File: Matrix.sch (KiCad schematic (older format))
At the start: 210 parts

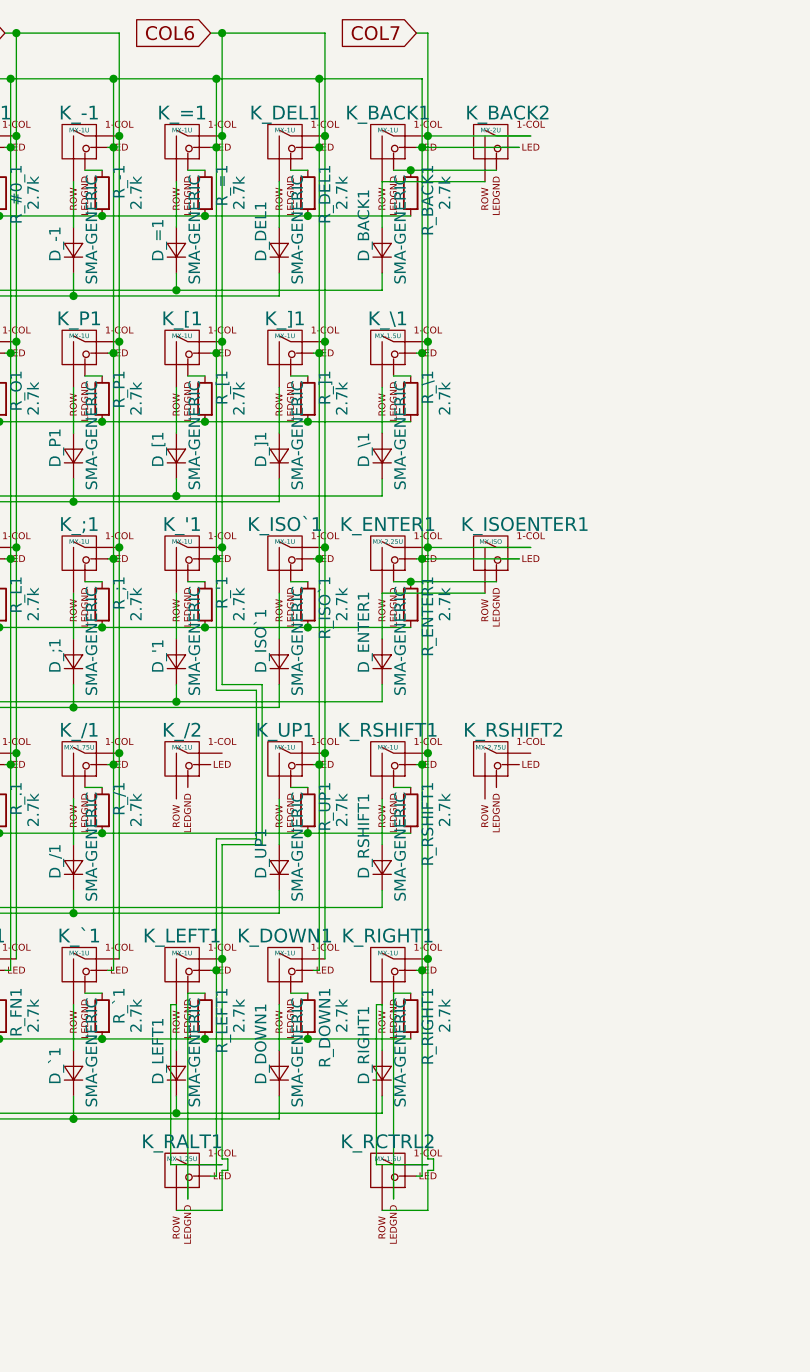
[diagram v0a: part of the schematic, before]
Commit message: Wire more LEDs
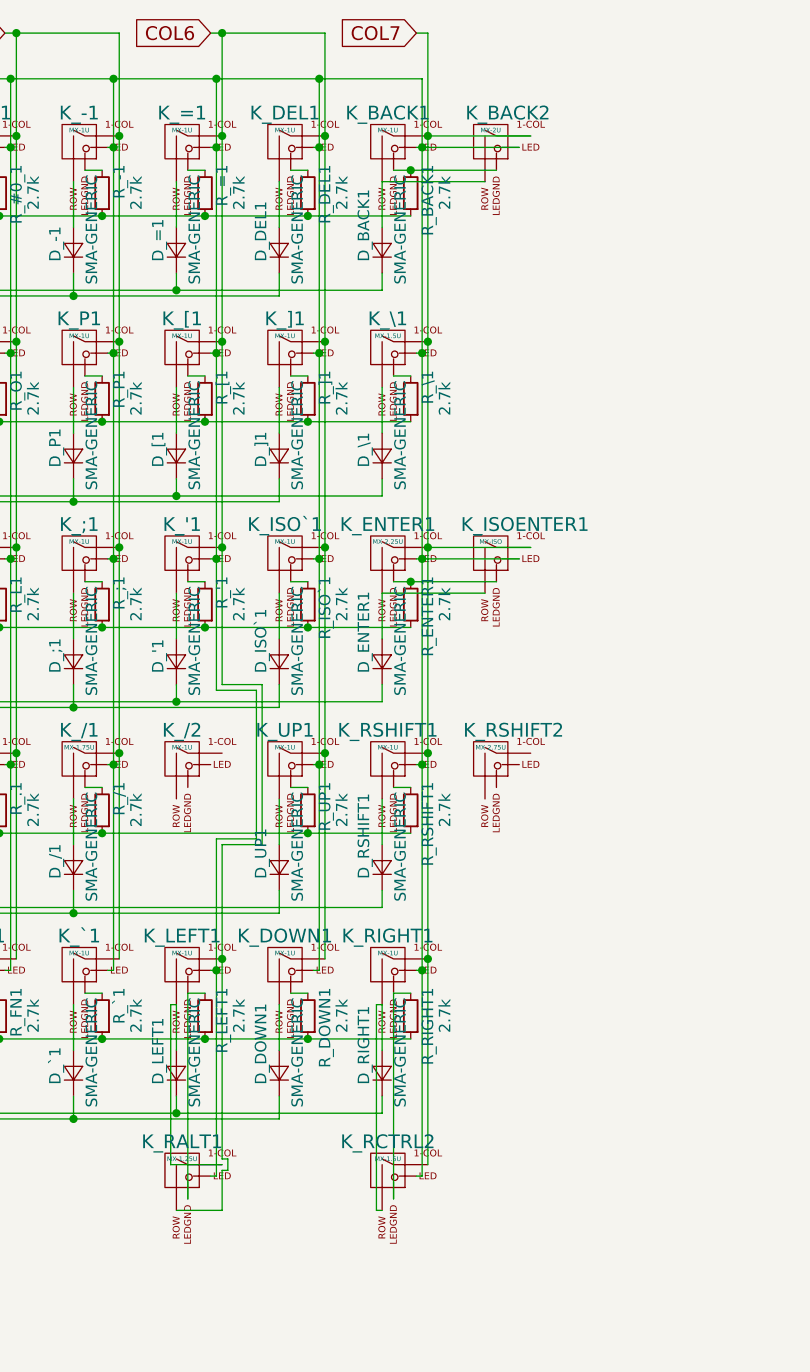
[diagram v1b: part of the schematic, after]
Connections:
- net COL7: now also K_RCTRL2.2 (COL); no longer K_RCTRL2.1 (ROW)
- net at D_RIGHT1.2 (A), K_RIGHT1.2 (ROW): now also K_RCTRL2.1 (ROW); no longer K_RCTRL2.2 (COL)
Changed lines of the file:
@@
 	9300 2150 9350 2150
 Wire Wire Line
-	9350 2150 9350 7075
+	9350 2150 9350 7100
 Connection ~ 9350 2600
 Connection ~ 9350 3500
@@
 	8425 7150 8400 7150
 Connection ~ 8425 6250
-Wire Wire Line
-	9150 7300 9350 7300
-Wire Wire Line
-	9350 7300 9350 7125
-Wire Wire Line
-	9350 7125 9375 7125
-Wire Wire Line
-	9375 7125 9375 7075
-Wire Wire Line
-	9375 7075 9350 7075
 Connection ~ 9350 6200
 Wire Wire Line
@@
 Connection ~ 9325 6250
 Wire Wire Line
-	9350 7100 9125 7100
-Wire Wire Line
-	9125 7100 9125 6400
+	9200 6350 9200 7250
+Wire Wire Line
+	9150 7300 9125 7300
+Wire Wire Line
+	9125 7300 9125 6400
 Wire Wire Line
 	9125 6400 9150 6400
-Wire Wire Line
-	9200 6350 9200 7250
 $EndSCHEMATC
